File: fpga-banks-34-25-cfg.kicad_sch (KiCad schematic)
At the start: 49 parts, among them J13 PinHeader_1x3_P2.54mm_Drill1.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, Q12 2N7002_SOT-23-3, Q13 2N7002_SOT-23-3, Q14 2N7002_SOT-23-3, Q15 2N7002_SOT-23-3, Q16 2N7002_SOT-23-3, U14 XC7A100T-FGG484

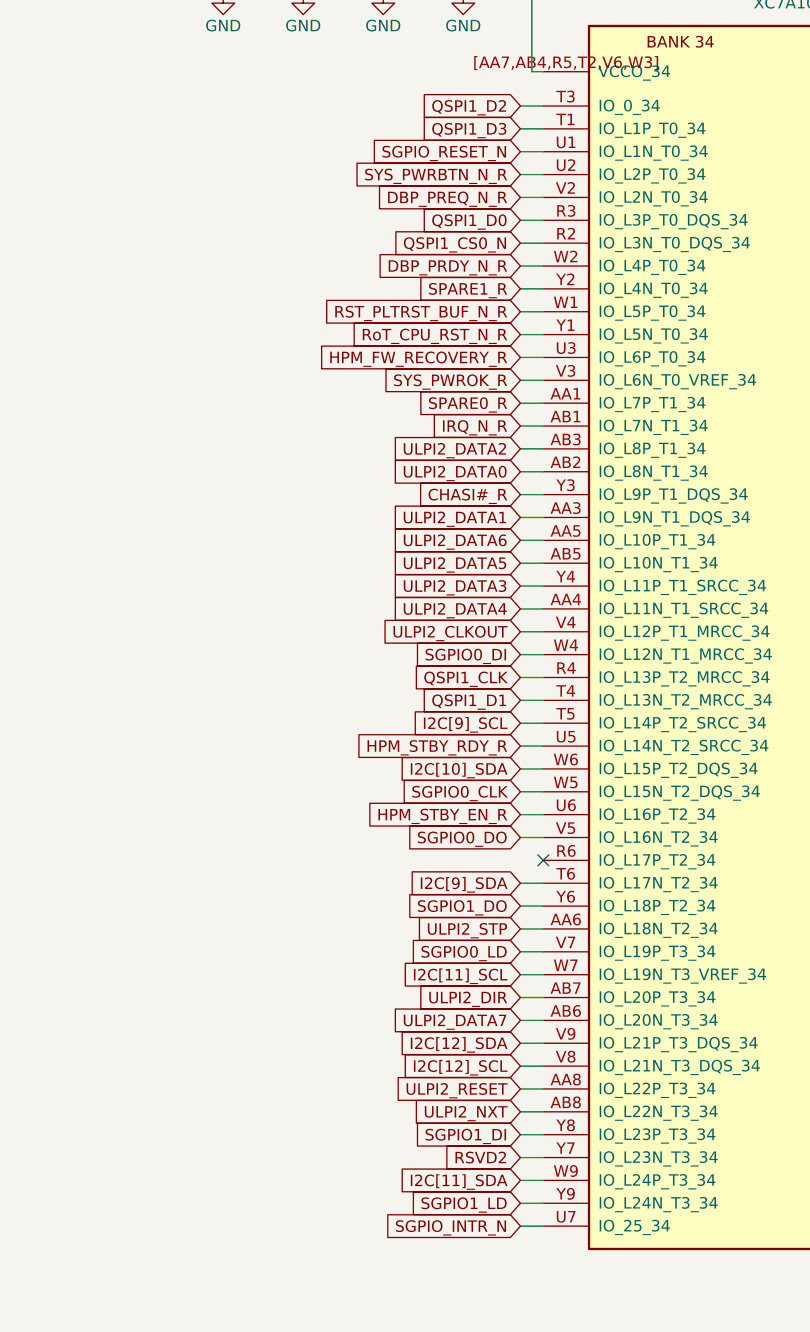
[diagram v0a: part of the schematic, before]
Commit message: river routing
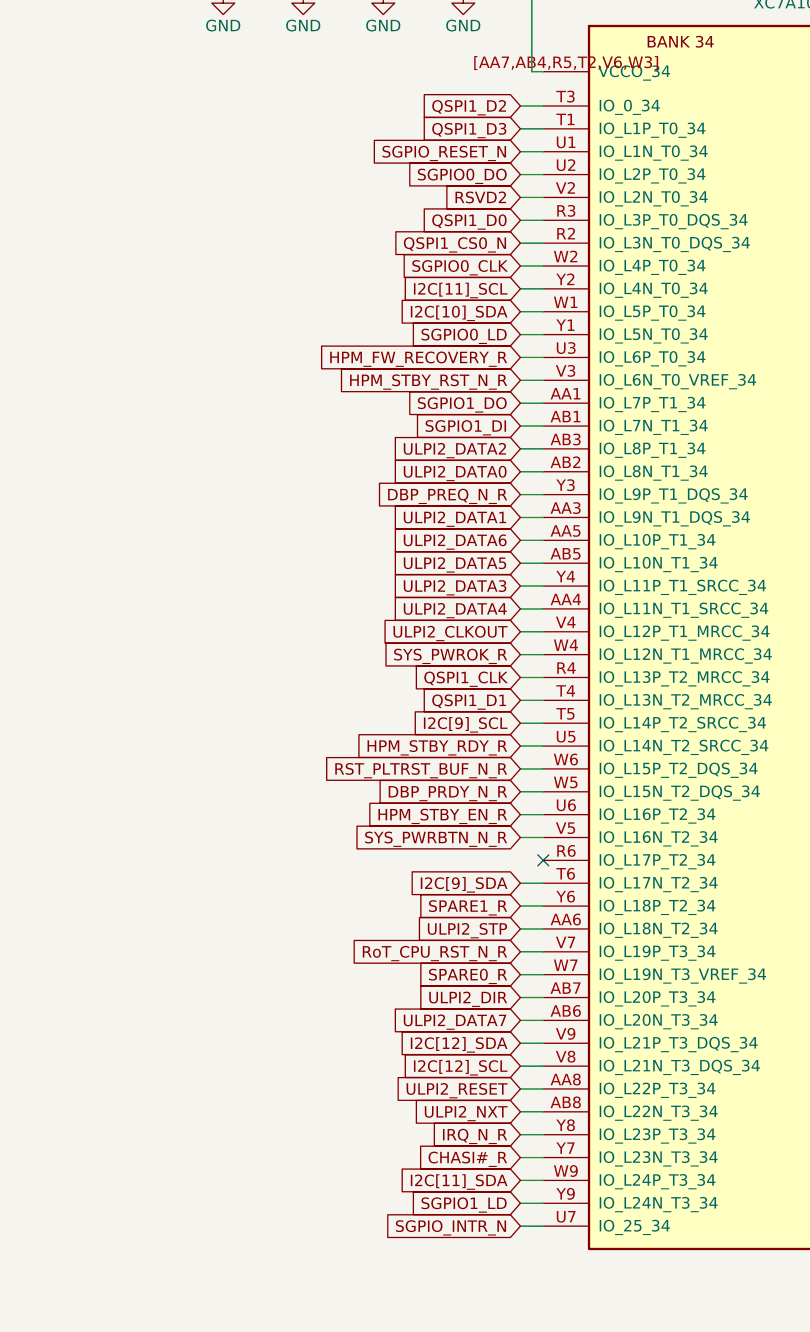
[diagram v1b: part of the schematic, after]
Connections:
- net SGPIO0_DI is gone; now on net SYS_PWROK_R: U14.W4 (IO_L12N_T1_MRCC_34)
- net CHASI#_R: now also U14.Y7 (IO_L23N_T3_34); no longer U14.Y3 (IO_L9P_T1_DQS_34)
- net DBP_PRDY_N_R: now also U14.W5 (IO_L15N_T2_DQS_34); no longer U14.W2 (IO_L4P_T0_34)
- net DBP_PREQ_N_R: now also U14.Y3 (IO_L9P_T1_DQS_34); no longer U14.V2 (IO_L2N_T0_34)
- net I2C[10]_SDA: now also U14.W1 (IO_L5P_T0_34); no longer U14.W6 (IO_L15P_T2_DQS_34)
- net I2C[11]_SCL: now also U14.Y2 (IO_L4N_T0_34); no longer U14.W7 (IO_L19N_T3_VREF_34)
- net IRQ_N_R: now also U14.Y8 (IO_L23P_T3_34); no longer U14.AB1 (IO_L7N_T1_34)
- net RST_PLTRST_BUF_N_R: now also U14.W6 (IO_L15P_T2_DQS_34); no longer U14.W1 (IO_L5P_T0_34)
- net RSVD2: now also U14.V2 (IO_L2N_T0_34); no longer U14.Y7 (IO_L23N_T3_34)
- net RoT_CPU_RST_N_R: now also U14.V7 (IO_L19P_T3_34); no longer U14.Y1 (IO_L5N_T0_34)
- net SGPIO0_CLK: now also U14.W2 (IO_L4P_T0_34); no longer U14.W5 (IO_L15N_T2_DQS_34)
- net SGPIO0_DO: now also U14.U2 (IO_L2P_T0_34); no longer U14.V5 (IO_L16N_T2_34)
- net SGPIO0_LD: now also U14.Y1 (IO_L5N_T0_34); no longer U14.V7 (IO_L19P_T3_34)
- net SGPIO1_DI: now also U14.AB1 (IO_L7N_T1_34); no longer U14.Y8 (IO_L23P_T3_34)
- net SGPIO1_DO: now also U14.AA1 (IO_L7P_T1_34); no longer U14.Y6 (IO_L18P_T2_34)
- net SPARE0_R: now also U14.W7 (IO_L19N_T3_VREF_34); no longer U14.AA1 (IO_L7P_T1_34)
- net SPARE1_R: now also U14.Y6 (IO_L18P_T2_34); no longer U14.Y2 (IO_L4N_T0_34)
- net SYS_PWRBTN_N_R: now also U14.V5 (IO_L16N_T2_34); no longer U14.U2 (IO_L2P_T0_34)
- net SYS_PWROK_R: no longer U14.V3 (IO_L6N_T0_VREF_34)
- new net HPM_STBY_RST_N_R: U14.V3 (IO_L6N_T0_VREF_34)

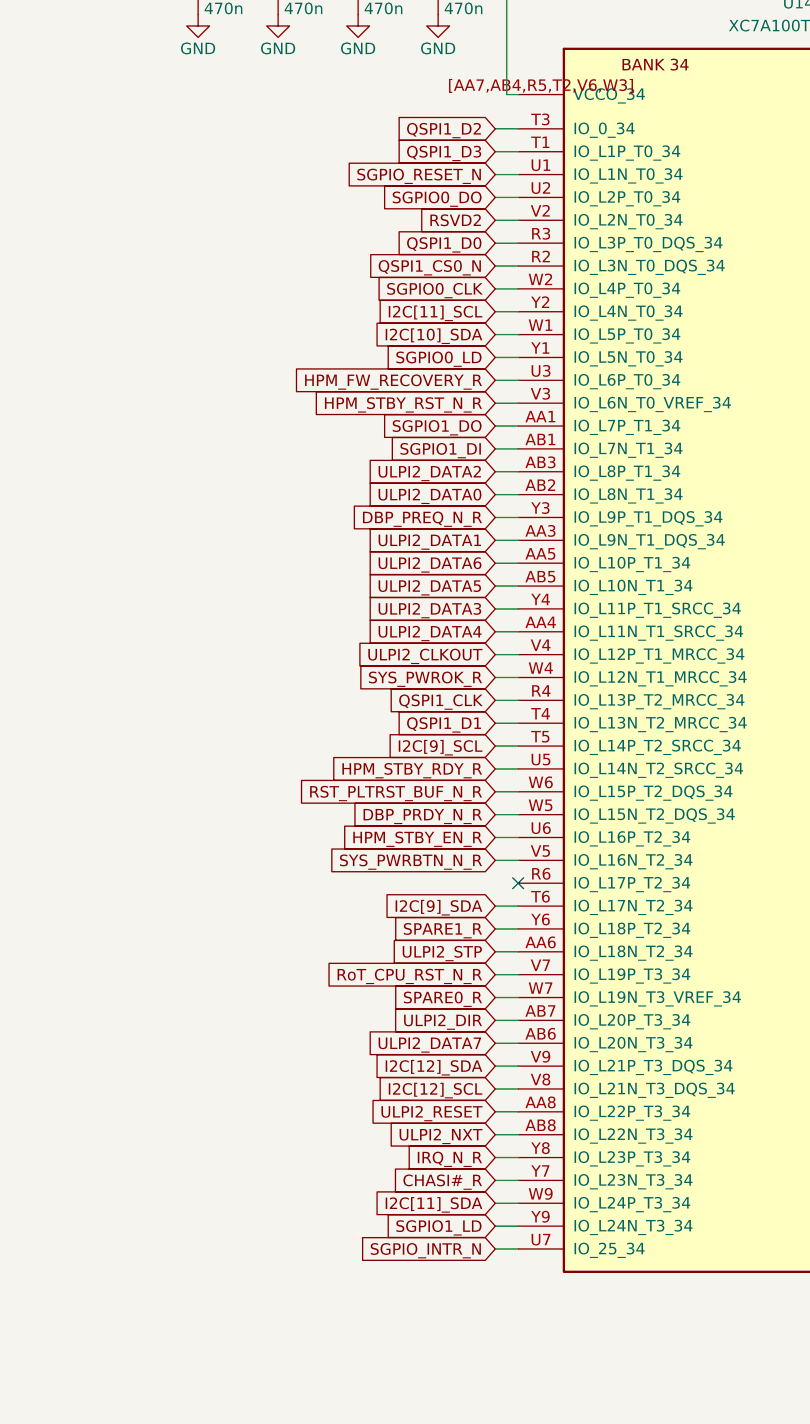
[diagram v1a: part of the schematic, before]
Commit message: Almost done with the routing
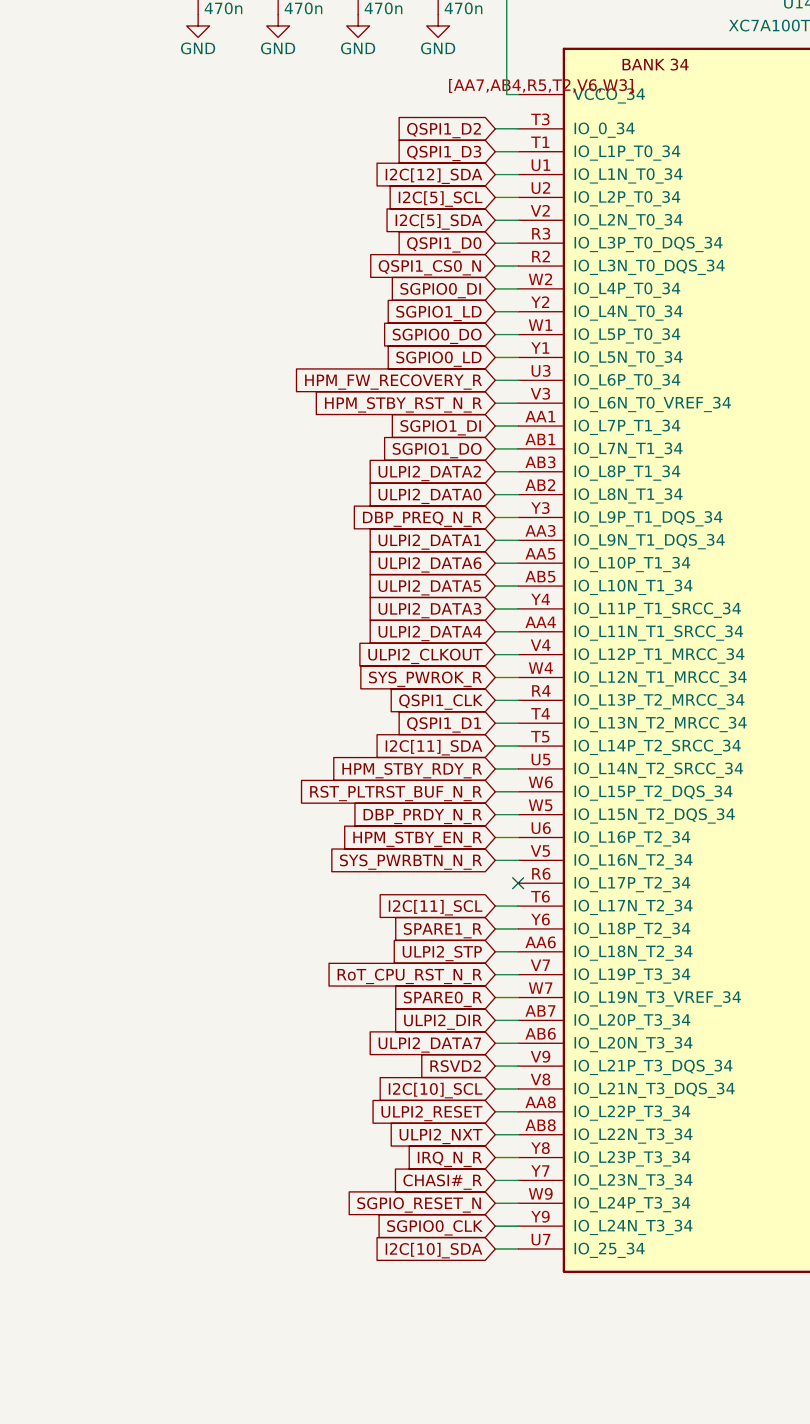
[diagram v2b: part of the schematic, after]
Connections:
- net I2C[9]_SCL is gone; now on net I2C[11]_SDA: U14.T5 (IO_L14P_T2_SRCC_34)
- net I2C[9]_SDA is gone; now on net I2C[11]_SCL: U14.T6 (IO_L17N_T2_34)
- net SGPIO_INTR_N is gone; now on net I2C[10]_SDA: U14.U7 (IO_25_34)
- net I2C[10]_SDA: no longer U14.W1 (IO_L5P_T0_34)
- net I2C[11]_SCL: no longer U14.Y2 (IO_L4N_T0_34)
- net I2C[11]_SDA: no longer U14.W9 (IO_L24P_T3_34)
- net I2C[12]_SDA: now also U14.U1 (IO_L1N_T0_34); no longer U14.V9 (IO_L21P_T3_DQS_34)
- net RSVD2: now also U14.V9 (IO_L21P_T3_DQS_34); no longer U14.V2 (IO_L2N_T0_34)
- net SGPIO0_CLK: now also U14.Y9 (IO_L24N_T3_34); no longer U14.W2 (IO_L4P_T0_34)
- net SGPIO0_DO: now also U14.W1 (IO_L5P_T0_34); no longer U14.U2 (IO_L2P_T0_34)
- net SGPIO1_DI: now also U14.AA1 (IO_L7P_T1_34); no longer U14.AB1 (IO_L7N_T1_34)
- net SGPIO1_DO: now also U14.AB1 (IO_L7N_T1_34); no longer U14.AA1 (IO_L7P_T1_34)
- net SGPIO1_LD: now also U14.Y2 (IO_L4N_T0_34); no longer U14.Y9 (IO_L24N_T3_34)
- net SGPIO_RESET_N: now also U14.W9 (IO_L24P_T3_34); no longer U14.U1 (IO_L1N_T0_34)
- net I2C[12]_SCL renamed I2C[10]_SCL
- new net I2C[5]_SCL: U14.U2 (IO_L2P_T0_34)
- new net I2C[5]_SDA: U14.V2 (IO_L2N_T0_34)
- new net SGPIO0_DI: U14.W2 (IO_L4P_T0_34)
